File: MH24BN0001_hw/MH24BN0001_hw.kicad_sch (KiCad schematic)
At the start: 7 parts, among them J1 ST-Link V2 Header, U1 STM32F401RBT6, U2 Accelerometer

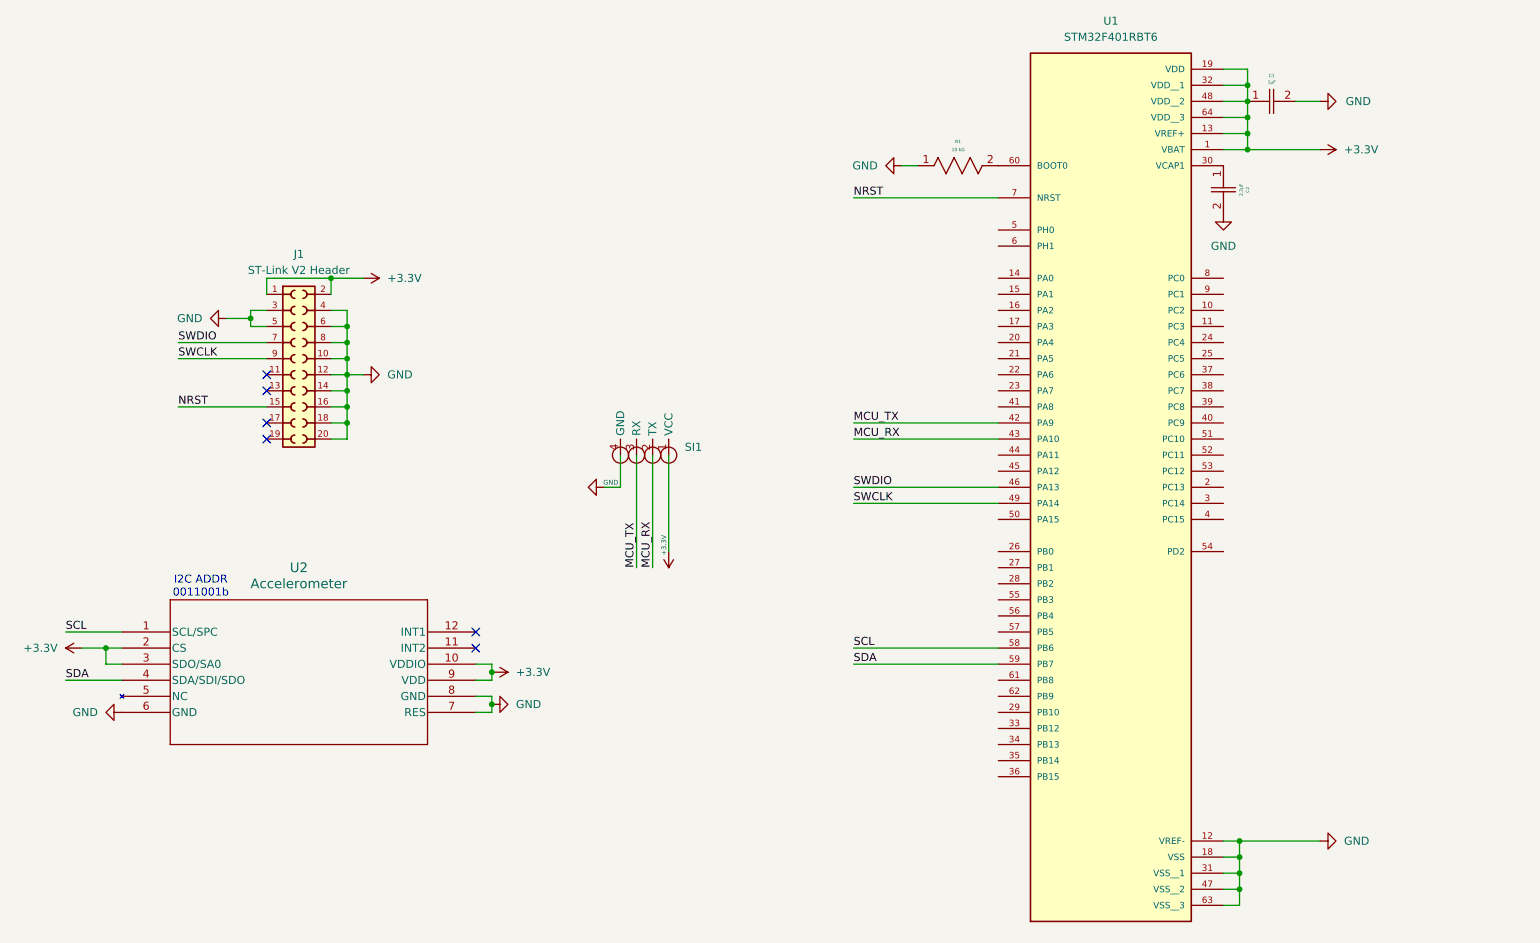
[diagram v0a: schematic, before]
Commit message: starting PCB
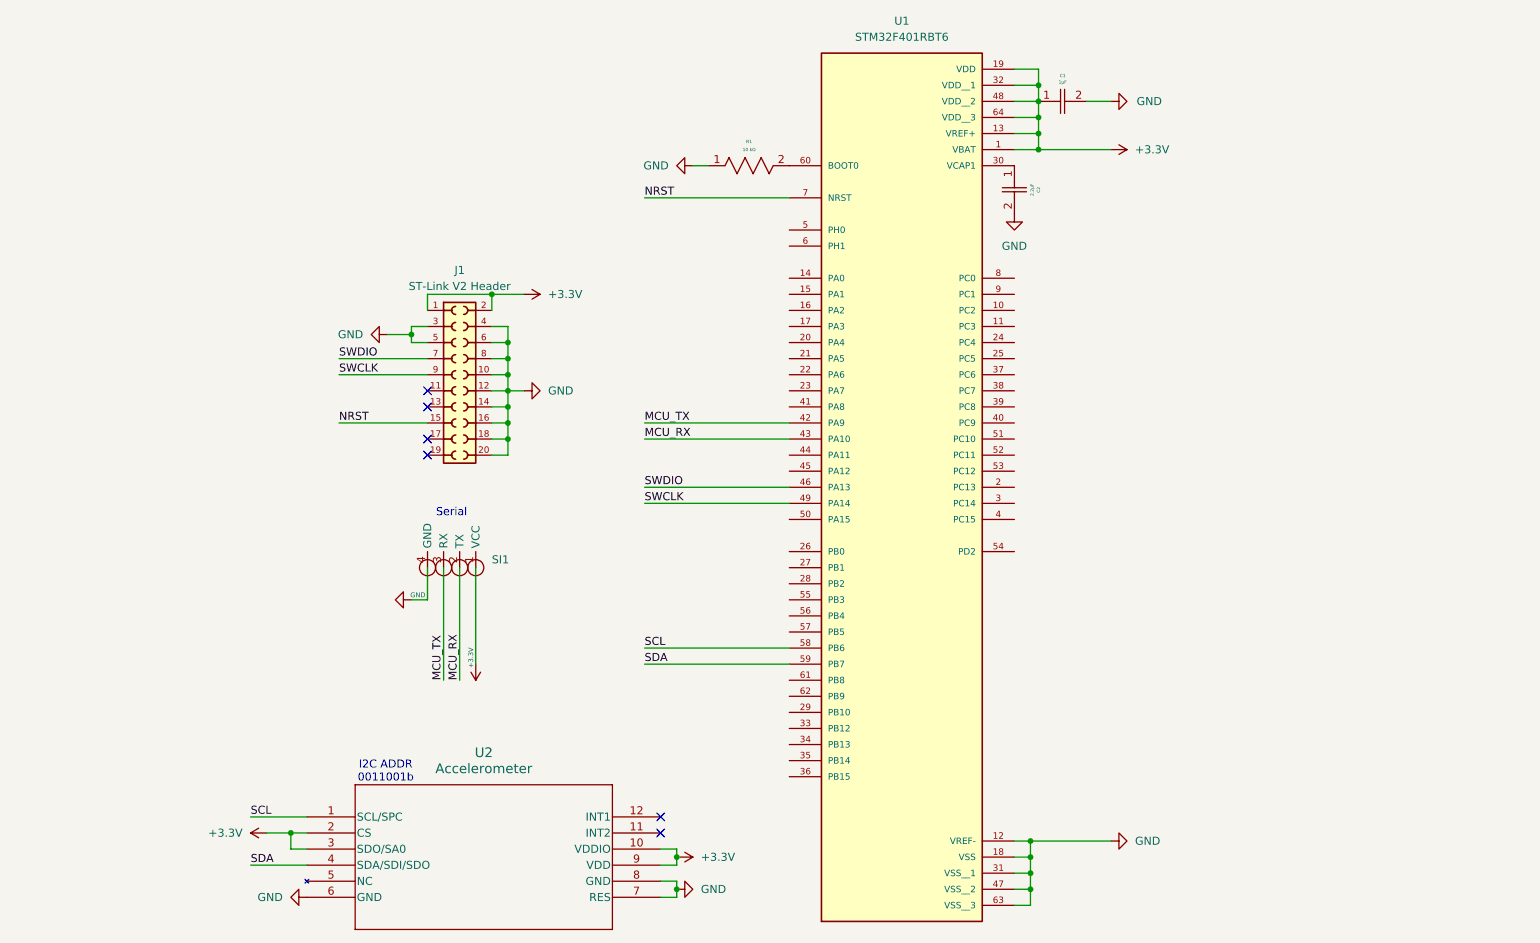
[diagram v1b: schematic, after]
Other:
- note added: "Serial"
- moved on the sheet: C1, C2, J1, R1, SI1, U1, U2

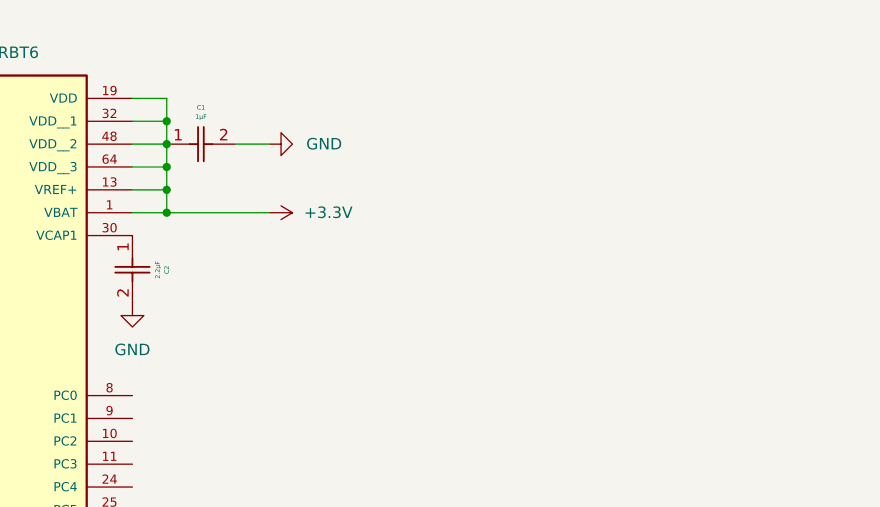
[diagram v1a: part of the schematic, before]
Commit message: finishing pcb, generating output files
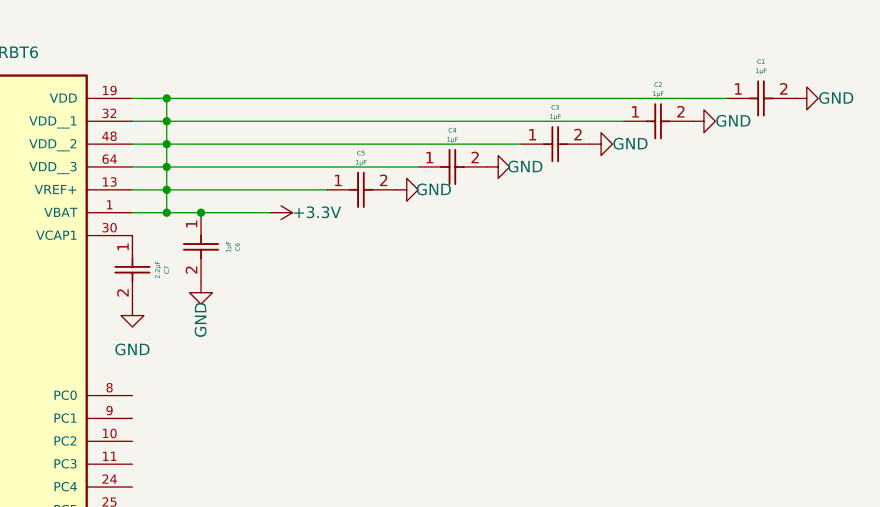
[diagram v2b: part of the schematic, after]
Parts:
- added C1, C2, C4, C5, C6: 1µF, Library:1µF_cap, symbol Sym_lib:CL10B105KP8NNNC
- renumbered C1 to C3, C2 to C7
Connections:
- net +3.3V: now also C1.1, C2.1, C4.1, C5.1, C6.1
- net GND: now also C1.2, C2.2, C4.2, C5.2, C6.2
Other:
- moved on the sheet: C3
